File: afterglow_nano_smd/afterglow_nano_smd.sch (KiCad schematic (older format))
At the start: 103 parts, among them J1 J137_IN_C, J2 J133_IN_R, J3 Conn_Power, J4 J133_OUT_R, J5 J137_OUT_C, J6 J134_OUT_R, J7 J138_OUT_C, J8 J135_OUT_R, J9 136_OUT_C, Q1 IRF5305, Q10 IRL2905, Q11 IRL2905, Q12 IRL2905, Q13 IRL2905, Q14 IRL2905, Q15 IRL2905, Q16 IRL2905, Q2 IRF5305, Q3 IRF5305, Q4 IRF5305, Q5 IRF5305, Q6 IRF5305, Q7 IRF5305, Q8 IRF5305, Q9 IRL2905, U1 74LS165, U2 74LS165, U3 5V_Regulator, U5 74HC595, U6 74HC595, U7 ULN2803A

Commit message: SMD version 1.3 preparations
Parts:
- removed R33, R34: 560, Resistors_SMD:R_0805_HandSoldering, symbol afterglow_nano_smd-rescue:R
- added JP1: Jumper, Pin_Headers:Pin_Header_Straight_1x02_Pitch2.54mm, symbol Device:Jumper
- added R26: 0.22, Resistors_SMD:R_0805_HandSoldering, symbol Device:R
- added R33, R34: 10k, Resistors_SMD:R_0805_HandSoldering, symbol Device:R
- added TP1, TP2, TP3: TestPoint, symbol Connector:TestPoint
- C4: symbol afterglow_nano_smd-rescue:C_Small -> Device:C_Small
- J1, J5, J7: footprint afterglow:Molex_KK-41791-9_9x3.96mm_Straight -> Connectors_Molex:Molex_KK-41791-9_9x3.96mm_Straight
- J3: symbol afterglow_nano_smd-rescue:Conn_01x02 -> Connector:Conn_01x02_Male
- Q1, Q2, Q3, Q4, Q5, Q6, Q7, Q8: symbol afterglow_nano_smd-rescue:IRF9540N -> Transistor_FET:IRF9540N
- Q10, Q11, Q12, Q13, Q14, Q15, Q16, Q9: symbol afterglow_nano_smd-rescue:IRF540N -> Transistor_FET:IRF540N
- R1, R2, R3, R4, R5, R6, R7, R8: value 390 -> 330
- R17, R25, R40, R41, R42, R43, R44, R45, R46, R47, R48, R49, R50, R51, R52, R53, R54, R55, R56, R57, R58, R59, R60, R61, R62, R63, R64, R65, R66: symbol afterglow_nano_smd-rescue:R -> Device:R
- R27, R28, R29, R30, R31, R32: value 560 -> 10k
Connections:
- net labels added: ROW_GND
- wire segments 242 -> 257
- no-connect marks 31 -> 30
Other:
- moved on the sheet: R10, R11, R12, R13, R14, R15, R16, R9, U2, U5, U6, U7

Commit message: FW upload preparations
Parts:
- R26: footprint Resistors_SMD:R_0805_HandSoldering -> Resistors_SMD:R_2512_HandSoldering
- TP1, TP2, TP3: footprint (none) -> Pin_Headers:Pin_Header_Straight_1x01_Pitch2.54mm
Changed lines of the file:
@@
 F 0 "R26" V 6100 1100 50  0000 C CNN
 F 1 "0.22" V 6200 1100 50  0000 C CNN
-F 2 "Resistors_SMD:R_0805_HandSoldering" V 6130 1100 50  0001 C CNN
+F 2 "Resistors_SMD:R_2512_HandSoldering" V 6130 1100 50  0001 C CNN
 F 3 "" H 6200 1100 50  0001 C CNN
 	1    6200 1100
@@
 F 0 "TP1" H 5758 3320 50  0000 L CNN
 F 1 "TestPoint" H 5758 3229 50  0000 L CNN
-F 2 "" H 5900 3200 50  0001 C CNN
+F 2 "Pin_Headers:Pin_Header_Straight_1x01_Pitch2.54mm" H 5900 3200 50  0001 C CNN
 F 3 "~" H 5900 3200 50  0001 C CNN
 	1    5700 3200
@@
 F 0 "TP2" H 6408 3320 50  0000 L CNN
 F 1 "TestPoint" H 6408 3229 50  0000 L CNN
-F 2 "" H 6550 3200 50  0001 C CNN
+F 2 "Pin_Headers:Pin_Header_Straight_1x01_Pitch2.54mm" H 6550 3200 50  0001 C CNN
 F 3 "~" H 6550 3200 50  0001 C CNN
 	1    6350 3200
@@
 F 0 "TP3" H 7058 3320 50  0000 L CNN
 F 1 "TestPoint" H 7058 3229 50  0000 L CNN
-F 2 "" H 7200 3200 50  0001 C CNN
+F 2 "Pin_Headers:Pin_Header_Straight_1x01_Pitch2.54mm" H 7200 3200 50  0001 C CNN
 F 3 "~" H 7200 3200 50  0001 C CNN
 	1    7000 3200

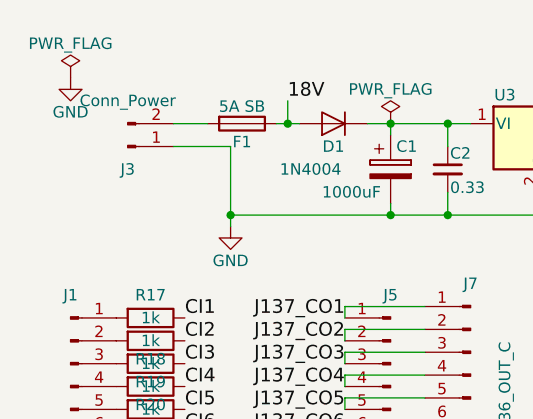
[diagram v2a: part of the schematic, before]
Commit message: v1.3 PCB progress
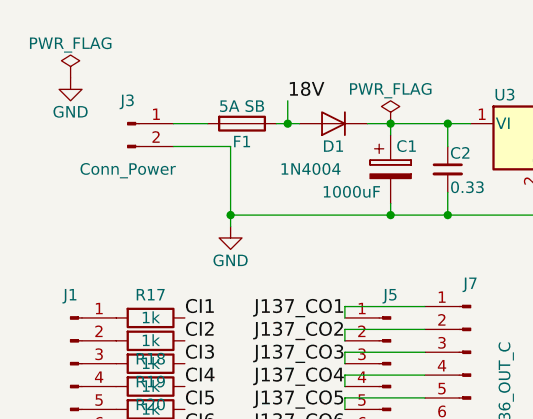
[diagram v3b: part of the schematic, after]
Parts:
- A1: footprint Module:Arduino_Nano -> Modules:Arduino_Nano
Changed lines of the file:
@@
 L Connector:Conn_01x02_Male J3
 U 1 1 59DA2DDC
-P 950 1100
-F 0 "J3" H 950 1200 50  0000 C CNN
-F 1 "Conn_Power" H 950 900 50  0000 C CNN
-F 2 "Connectors_Molex:Molex_KK-41791-02_02x3.96mm_Straight" H 950 1100 50  0001 C CNN
-F 3 "" H 950 1100 50  0001 C CNN
-	1    950  1100
-	1    0    0    1
+P 950 1000
+F 0 "J3" H 950 1100 50  0000 C CNN
+F 1 "Conn_Power" H 950 800 50  0000 C CNN
+F 2 "Connectors_Molex:Molex_KK-41791-02_02x3.96mm_Straight" H 950 1000 50  0001 C CNN
+F 3 "" H 950 1000 50  0001 C CNN
+	1    950  1000
+	1    0    0    -1
 $EndComp
 NoConn ~ 900  2550
@@
 F 0 "A1" H 3850 1250 50  0000 C CNN
 F 1 "Arduino_Nano_v3.x" H 3850 1150 50  0000 C CNN
-F 2 "Module:Arduino_Nano" H 4500 1400 50  0001 L CNN
+F 2 "Modules:Arduino_Nano" H 4500 1400 50  0001 L CNN
 F 3 "http://www.mouser.com/pdfdocs/Gravitech_Arduino_Nano3_0.pdf" H 4350 1350 50  0001 C CNN
 	1    4350 2350

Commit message: v1.3 progressing
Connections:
- net labels added: SUP_GND
- net labels removed: ROW_GND
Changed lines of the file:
@@
 Connection ~ 6000 1100
 Text Label 6000 950  0    60   ~ 0
-ROW_GND
+SUP_GND
 Wire Wire Line
 	10300 1050 10300 1150
@@
 Connection ~ 10300 6300
 Text Label 10300 1900 0    60   ~ 0
-ROW_GND
+SUP_GND
 Text Label 10300 2650 0    60   ~ 0
-ROW_GND
+SUP_GND
 Text Label 10300 3400 0    60   ~ 0
-ROW_GND
+SUP_GND
 Text Label 10300 4150 0    60   ~ 0
-ROW_GND
+SUP_GND
 Text Label 10300 4900 0    60   ~ 0
-ROW_GND
+SUP_GND
 Text Label 10300 5650 0    60   ~ 0
-ROW_GND
+SUP_GND
 Text Label 10300 6400 0    60   ~ 0
-ROW_GND
+SUP_GND
 Text Label 10300 1150 0    60   ~ 0
-ROW_GND
+SUP_GND
 Wire Wire Line
 	6000 1100 6000 2350
@@
 Connection ~ 8200 1050
 $Comp
-L power:GND #PWR03
-U 1 1 5BA996DF
-P 7900 1050
-F 0 "#PWR03" H 7900 800 50  0001 C CNN
-F 1 "GND" H 7905 877 50  0000 C CNN
-F 2 "" H 7900 1050 50  0001 C CNN
-F 3 "" H 7900 1050 50  0001 C CNN
-	1    7900 1050
-	1    0    0    -1
-$EndComp
-$Comp
 L Device:R R28
 U 1 1 5BA99EBD
@@
 Connection ~ 8200 3300
 $Comp
-L power:GND #PWR04
-U 1 1 5BA9A69A
-P 7900 1800
-F 0 "#PWR04" H 7900 1550 50  0001 C CNN
-F 1 "GND" H 7905 1627 50  0000 C CNN
-F 2 "" H 7900 1800 50  0001 C CNN
-F 3 "" H 7900 1800 50  0001 C CNN
-	1    7900 1800
-	1    0    0    -1
-$EndComp
-$Comp
-L power:GND #PWR05
-U 1 1 5BA9A77D
-P 7900 2550
-F 0 "#PWR05" H 7900 2300 50  0001 C CNN
-F 1 "GND" H 7905 2377 50  0000 C CNN
-F 2 "" H 7900 2550 50  0001 C CNN
-F 3 "" H 7900 2550 50  0001 C CNN
-	1    7900 2550
-	1    0    0    -1
-$EndComp
-$Comp
-L power:GND #PWR06
-U 1 1 5BA9AA10
-P 7900 3300
-F 0 "#PWR06" H 7900 3050 50  0001 C CNN
-F 1 "GND" H 7905 3127 50  0000 C CNN
-F 2 "" H 7900 3300 50  0001 C CNN
-F 3 "" H 7900 3300 50  0001 C CNN
-	1    7900 3300
-	1    0    0    -1
-$EndComp
-$Comp
 L Device:R R31
 U 1 1 5BA9ADD5
@@
 Connection ~ 8200 4050
 $Comp
-L power:GND #PWR07
-U 1 1 5BA9AEEF
-P 7900 4050
-F 0 "#PWR07" H 7900 3800 50  0001 C CNN
-F 1 "GND" H 7905 3877 50  0000 C CNN
-F 2 "" H 7900 4050 50  0001 C CNN
-F 3 "" H 7900 4050 50  0001 C CNN
-	1    7900 4050
-	1    0    0    -1
-$EndComp
-$Comp
 L Device:R R32
 U 1 1 5BA9B262
@@
 Connection ~ 8250 6300
 $Comp
-L power:GND #PWR08
-U 1 1 5BA9BE49
-P 7900 4800
-F 0 "#PWR08" H 7900 4550 50  0001 C CNN
-F 1 "GND" H 7905 4627 50  0000 C CNN
-F 2 "" H 7900 4800 50  0001 C CNN
-F 3 "" H 7900 4800 50  0001 C CNN
-	1    7900 4800
-	1    0    0    -1
-$EndComp
-$Comp
-L power:GND #PWR09
-U 1 1 5BA9C1D4
-P 7900 5550
-F 0 "#PWR09" H 7900 5300 50  0001 C CNN
-F 1 "GND" H 7905 5377 50  0000 C CNN
-F 2 "" H 7900 5550 50  0001 C CNN
-F 3 "" H 7900 5550 50  0001 C CNN
-	1    7900 5550
-	1    0    0    -1
-$EndComp
-$Comp
-L power:GND #PWR011
-U 1 1 5BA9C39F
-P 7950 6300
-F 0 "#PWR011" H 7950 6050 50  0001 C CNN
-F 1 "GND" H 7955 6127 50  0000 C CNN
-F 2 "" H 7950 6300 50  0001 C CNN
-F 3 "" H 7950 6300 50  0001 C CNN
-	1    7950 6300
-	1    0    0    -1
-$EndComp
-$Comp
 L Device:Jumper JP1
 U 1 1 5BAB0DAE
@@
 Text Label 7000 3200 2    60   ~ 0
 18V
+Text Label 7900 1050 2    60   ~ 0
+SUP_GND
+Text Label 7900 1800 2    60   ~ 0
+SUP_GND
+Text Label 7900 2550 2    60   ~ 0
+SUP_GND
+Text Label 7900 3300 2    60   ~ 0
+SUP_GND
+Text Label 7900 4050 2    60   ~ 0
+SUP_GND
+Text Label 7900 4800 2    60   ~ 0
+SUP_GND
+Text Label 7900 5550 2    60   ~ 0
+SUP_GND
+Text Label 7950 6300 2    60   ~ 0
+SUP_GND
 $EndSCHEMATC
